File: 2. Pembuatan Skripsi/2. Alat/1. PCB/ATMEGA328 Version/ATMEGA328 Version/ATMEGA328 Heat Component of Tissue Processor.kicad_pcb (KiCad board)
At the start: 2 copper layers, 52.3 x 63.6 mm, 64 parts, among them J1 Conn_01x02, J2 Sensors, J3 Screw_Terminal_01x02, J5 FTDI, J6 Conn_02x04_Top_Bottom, K1 EE2-4.5NU, Q1 S9013, Q2 S9013, Q3 S9013, Q4 MMBT2222, SW1 SW_SPST, SW2 SW_SPST, SW3 SW_SPST, U2 AP2112K-3.3, U3 ATmega328P-A, Y1 16MHz

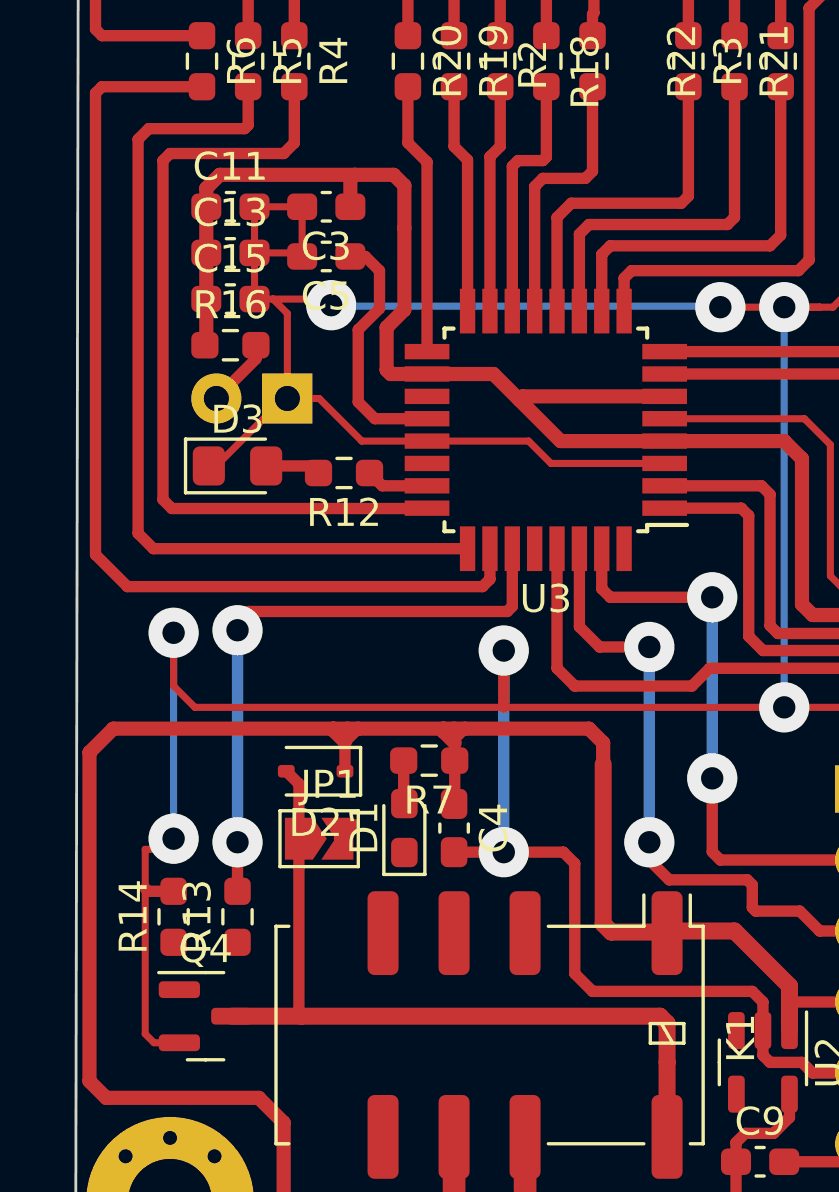
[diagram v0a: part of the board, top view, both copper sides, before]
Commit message: Huge Update
- New program
- Report updated
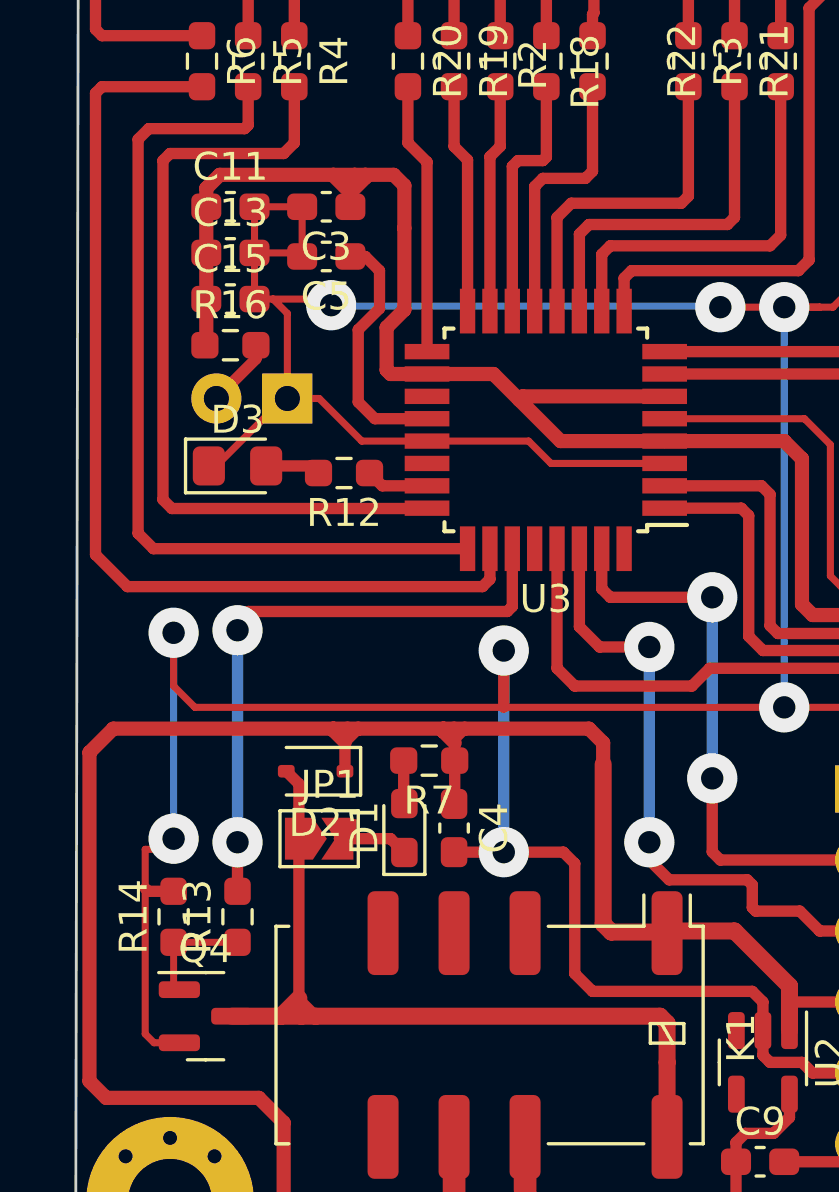
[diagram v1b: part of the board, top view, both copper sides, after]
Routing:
- net Net-(Q4-B): track 0.00 -> 4.06 mm
- net Net-(D1-K): track 0.72 -> 3.25 mm
- net Opto: track 28.7 -> 30.5 mm
- net VCC: track 319.3 -> 321.0 mm
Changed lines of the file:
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@@
   (segment (start 55.499 119.507) (end 54.901957 118.909957) (width 0.508) (layer "F.Cu") (net 1))
   (segment (start 64.042 106.934) (end 64.042 106.773) (width 0.4064) (layer "F.Cu") (net 1))
+  (segment (start 64.2355 87.63) (end 64.2355 87.122) (width 0.508) (layer "F.Cu") (net 1))
   (segment (start 103.104 93.8405) (end 103.357296 93.8405) (width 0.6096) (layer "F.Cu") (net 1))
   (segment (start 67.9685 106.807) (end 67.9685 106.3225) (width 0.4064) (layer "F.Cu") (net 1))
@@
   (segment (start 59.563 86.487) (end 59.0815 86.9685) (width 0.508) (layer "F.Cu") (net 1))
   (segment (start 75.478 94.412) (end 70.396 94.412) (width 0.508) (layer "F.Cu") (net 1))
-  (segment (start 65.786 86.487) (end 64.389 86.487) (width 0.508) (layer "F.Cu") (net 1))
   (segment (start 103.38211 103.759) (end 103.382878 103.759) (width 0.6096) (layer "F.Cu") (net 1))
   (segment (start 89.027 104.267) (end 88.6695 104.6245) (width 0.6096) (layer "F.Cu") (net 1))
@@
   (segment (start 99.822 118.999) (end 102.87 118.999) (width 0.6096) (layer "F.Cu") (net 1))
   (segment (start 75.245234 126.049908) (end 62.39806 126.02506) (width 0.508) (layer "F.Cu") (net 1))
+  (segment (start 64.77 86.487) (end 64.77 86.5875) (width 0.508) (layer "F.Cu") (net 1))
   (segment (start 95.9955 84.5655) (end 98.659 84.5655) (width 0.6096) (layer "F.Cu") (net 1))
   (segment (start 94.742 80.518) (end 85.659 80.518) (width 0.4064) (layer "F.Cu") (net 1))
@@
   (segment (start 68.326 106.299) (end 67.945 106.299) (width 0.508) (layer "F.Cu") (net 1))
   (segment (start 98.659 84.5655) (end 103.231 84.5655) (width 0.6096) (layer "F.Cu") (net 1))
+  (segment (start 63.627 86.5135) (end 64.2355 87.122) (width 0.508) (layer "F.Cu") (net 1))
   (segment (start 95.377 83.947) (end 95.9955 84.5655) (width 0.6096) (layer "F.Cu") (net 1))
   (segment (start 75.603 113.538) (end 77.978 113.538) (width 0.6096) (layer "F.Cu") (net 1))
@@
   (segment (start 79.756 96.012) (end 80.391 96.647) (width 0.508) (layer "F.Cu") (net 1))
   (segment (start 73.279 106.807) (end 72.771 106.299) (width 0.508) (layer "F.Cu") (net 1))
+  (segment (start 63.627 86.487) (end 63.627 86.5135) (width 0.508) (layer "F.Cu") (net 1))
   (segment (start 64.3625 87.503) (end 64.2355 87.63) (width 0.508) (layer "F.Cu") (net 1))
   (segment (start 103.378 103.759) (end 92.719288 103.759) (width 0.6096) (layer "F.Cu") (net 1))
   (segment (start 103.357296 93.8405) (end 103.357296 93.78719) (width 0.6096) (layer "F.Cu") (net 1))
   (segment (start 72.771 106.299) (end 68.326 106.299) (width 0.508) (layer "F.Cu") (net 1))
+  (segment (start 64.2355 87.122) (end 64.2355 86.6405) (width 0.508) (layer "F.Cu") (net 1))
   (segment (start 100.004 93.8405) (end 103.104 93.8405) (width 0.6096) (layer "F.Cu") (net 1))
   (segment (start 90.551 102.235) (end 91.1606 101.6254) (width 0.508) (layer "F.Cu") (net 1))
@@
   (segment (start 95.4005 81.1765) (end 94.742 80.518) (width 0.4064) (layer "F.Cu") (net 1))
   (segment (start 67.9685 106.807) (end 67.9685 106.6565) (width 0.4064) (layer "F.Cu") (net 1))
+  (segment (start 63.627 86.487) (end 59.563 86.487) (width 0.508) (layer "F.Cu") (net 1))
   (segment (start 73.279 113.284) (end 73.571 113.576) (width 0.6096) (layer "F.Cu") (net 1))
   (segment (start 92.719288 103.759) (end 92.211288 104.267) (width 0.6096) (layer "F.Cu") (net 1))
@@
   (segment (start 99.187 124.968) (end 99.187 119.634) (width 0.6096) (layer "F.Cu") (net 1))
   (segment (start 67.9685 107.442) (end 67.9685 108.969) (width 0.4064) (layer "F.Cu") (net 1))
+  (segment (start 64.389 86.487) (end 63.627 86.487) (width 0.508) (layer "F.Cu") (net 1))
   (segment (start 104.017878 103.124) (end 104.01711 103.759) (width 0.6096) (layer "F.Cu") (net 1))
   (segment (start 104.041355 76.355355) (end 104.041355 83.7165) (width 0.6096) (layer "F.Cu") (net 1))
@@
   (segment (start 79.944 116.078) (end 79.944 117.0995) (width 0.4064) (layer "F.Cu") (net 1))
   (segment (start 95.4005 81.1765) (end 95.377 81.2) (width 0.6096) (layer "F.Cu") (net 1))
+  (segment (start 65.786 86.487) (end 64.77 86.487) (width 0.508) (layer "F.Cu") (net 1))
   (segment (start 65.672 93.612) (end 66.978 93.612) (width 0.508) (layer "F.Cu") (net 1))
   (segment (start 64.516 106.299) (end 67.564 106.299) (width 0.508) (layer "F.Cu") (net 1))
   (segment (start 61.849 120.396) (end 60.96 119.507) (width 0.508) (layer "F.Cu") (net 1))
   (segment (start 95.377 87.122) (end 95.377 85.217) (width 0.508) (layer "F.Cu") (net 1))
-  (segment (start 64.2355 87.63) (end 64.2355 86.6405) (width 0.508) (layer "F.Cu") (net 1))
+  (segment (start 64.77 86.487) (end 64.389 86.487) (width 0.508) (layer "F.Cu") (net 1))
   (segment (start 104.01711 104.394) (end 104.01711 103.759) (width 0.6096) (layer "F.Cu") (net 1))
   (segment (start 77.978 113.538) (end 79.944 115.504) (width 0.6096) (layer "F.Cu") (net 1))
@@
   (segment (start 104.028296 94.5115) (end 104.017878 103.124) (width 0.6096) (layer "F.Cu") (net 1))
   (segment (start 103.357296 93.8405) (end 104.028296 94.5115) (width 0.6096) (layer "F.Cu") (net 1))
+  (segment (start 64.77 86.5875) (end 64.2355 87.122) (width 0.508) (layer "F.Cu") (net 1))
   (segment (start 103.938218 93.8405) (end 104.029218 93.7495) (width 0.6096) (layer "F.Cu") (net 1))
   (segment (start 93.848722 126.049908) (end 75.245234 126.049908) (width 0.508) (layer "F.Cu") (net 1))
@@
   (segment (start 66.167 91.313) (end 65.532 91.948) (width 0.508) (layer "F.Cu") (net 1))
   (segment (start 75.478 96.012) (end 79.756 96.012) (width 0.508) (layer "F.Cu") (net 1))
-  (segment (start 64.389 86.487) (end 59.563 86.487) (width 0.508) (layer "F.Cu") (net 1))
   (segment (start 67.9685 106.6565) (end 68.326 106.299) (width 0.4064) (layer "F.Cu") (net 1))
   (segment (start 88.6695 104.6245) (end 88.6695 105.537) (width 0.6096) (layer "F.Cu") (net 1))
@@
   (segment (start 64.516 92.030054) (end 65.278 91.268054) (width 0.4064) (layer "F.Cu") (net 3))
   (segment (start 64.516 94.615) (end 64.516 92.030054) (width 0.4064) (layer "F.Cu") (net 3))
+  (segment (start 65.673 110.236) (end 66.167 110.73) (width 0.4064) (layer "F.Cu") (net 4))
+  (segment (start 63.844 110.236) (end 65.673 110.236) (width 0.4064) (layer "F.Cu") (net 4))
   (segment (start 64.352 109.728) (end 63.844 110.236) (width 0.4064) (layer "F.Cu") (net 4))
   (segment (start 66.1435 108.9565) (end 66.167 108.98) (width 0.4064) (layer "F.Cu") (net 5))
   (segment (start 66.1435 107.442) (end 66.1435 108.9565) (width 0.4064) (layer "F.Cu") (net 5))
   (segment (start 62.394 116.496) (end 62.484 116.586) (width 0.4064) (layer "F.Cu") (net 6))
-  (segment (start 62.394 110.236) (end 62.394 116.496) (width 0.4064) (layer "F.Cu") (net 6))
+  (segment (start 61.722 116.586) (end 62.484 116.586) (width 0.6096) (layer "F.Cu") (net 6))
+  (segment (start 62.394 115.988) (end 62.992 116.586) (width 0.4064) (layer "F.Cu") (net 6))
+  (segment (start 62.484 116.586) (end 62.992 116.586) (width 0.6096) (layer "F.Cu") (net 6))
   (segment (start 75.565 116.84) (end 75.565 118.237) (width 0.6096) (layer "F.Cu") (net 6))
+  (segment (start 62.394 115.951) (end 62.394 116.496) (width 0.4064) (layer "F.Cu") (net 6))
+  (segment (start 61.759 116.586) (end 62.394 115.951) (width 0.6096) (layer "F.Cu") (net 6))
   (segment (start 62.394 108.275) (end 61.942 107.823) (width 0.4064) (layer "F.Cu") (net 6))
-  (segment (start 62.484 116.586) (end 75.311 116.586) (width 0.6096) (layer "F.Cu") (net 6))
+  (segment (start 59.9925 116.586) (end 61.722 116.586) (width 0.6096) (layer "F.Cu") (net 6))
   (segment (start 62.394 110.236) (end 62.394 108.275) (width 0.4064) (layer "F.Cu") (net 6))
+  (segment (start 62.992 116.586) (end 75.311 116.586) (width 0.6096) (layer "F.Cu") (net 6))
+  (segment (start 62.394 115.951) (end 62.394 115.988) (width 0.4064) (layer "F.Cu") (net 6))
+  (segment (start 62.394 110.236) (end 62.394 115.951) (width 0.4064) (layer "F.Cu") (net 6))
   (segment (start 75.565 118.237) (end 75.565 120.866) (width 0.6096) (layer "F.Cu") (net 6))
   (segment (start 75.311 116.586) (end 75.565 116.84) (width 0.6096) (layer "F.Cu") (net 6))
-  (segment (start 59.9925 116.586) (end 62.484 116.586) (width 0.6096) (layer "F.Cu") (net 6))
+  (segment (start 61.722 116.586) (end 61.759 116.586) (width 0.6096) (layer "F.Cu") (net 6))
   (segment (start 60.8565 93.0725) (end 59.441 94.488) (width 0.4064) (layer "F.Cu") (net 7))
   (segment (start 60.8565 92.583) (end 60.8565 93.0725) (width 0.4064) (layer "F.Cu") (net 7))
@@
   (segment (start 72.009 69.088) (end 78.232 69.088) (width 0.4064) (layer "F.Cu") (net 26))
   (segment (start 71.374 65.913) (end 71.628 66.167) (width 0.4064) (layer "F.Cu") (net 26))
+  (segment (start 57.912 115.4305) (end 58.1175 115.636) (width 0.25) (layer "F.Cu") (net 27))
+  (segment (start 57.912 113.9425) (end 57.912 115.4305) (width 0.25) (layer "F.Cu") (net 27))
+  (segment (start 57.912 113.9425) (end 60.198 113.9425) (width 0.25) (layer "F.Cu") (net 27))
   (segment (start 90.658 77.2395) (end 89.896 78.0015) (width 0.4064) (layer "F.Cu") (net 28))
   (segment (start 90.658 65.6825) (end 90.658 77.2395) (width 0.4064) (layer "F.Cu") (net 28))
